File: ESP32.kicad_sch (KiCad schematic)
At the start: 4 parts, among them U1 ESP32-S3

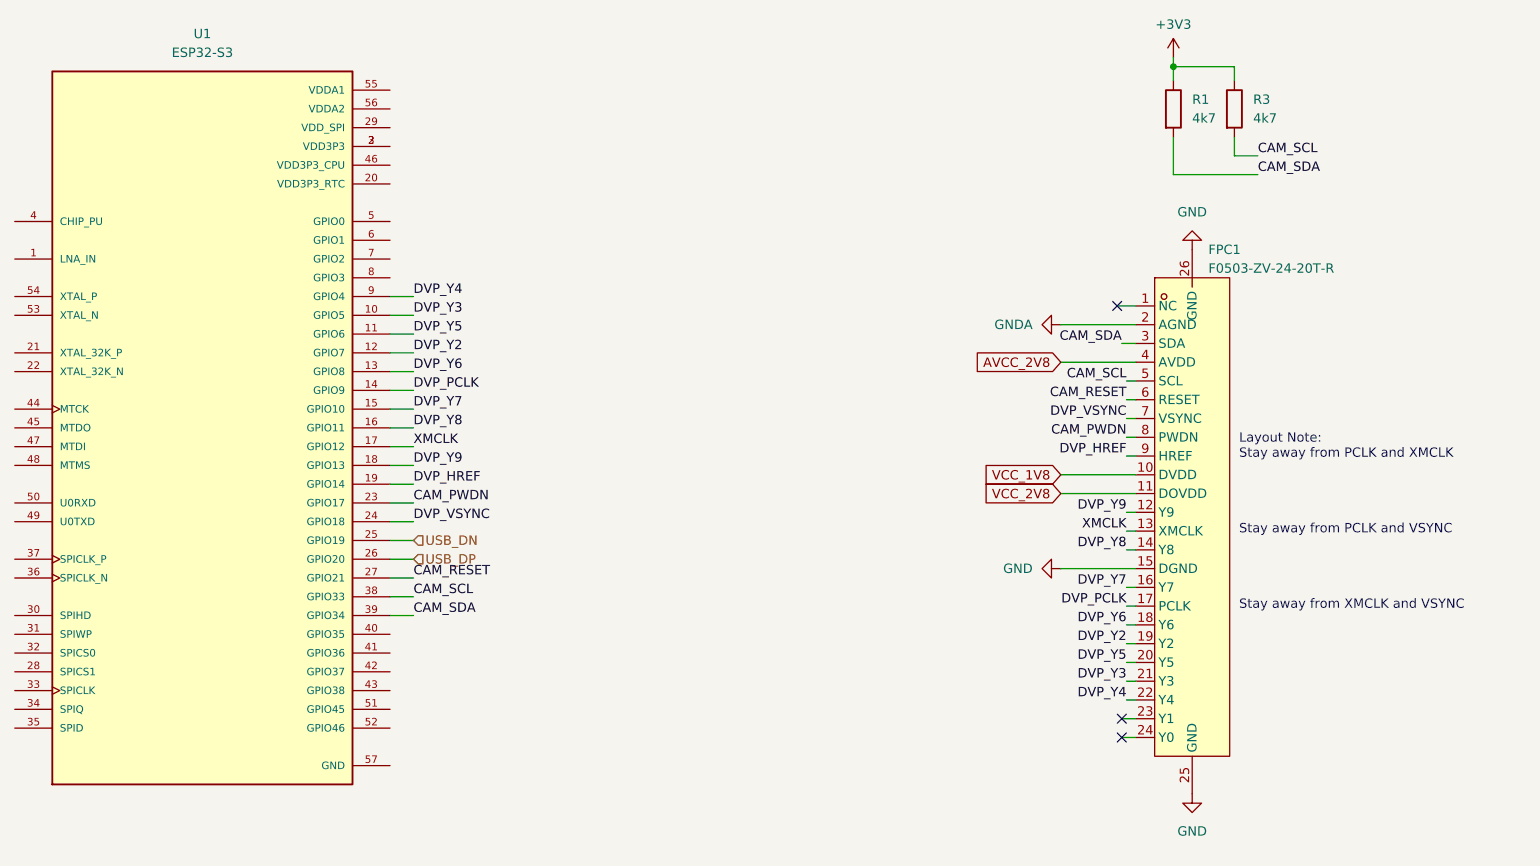
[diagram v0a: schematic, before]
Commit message: revving up
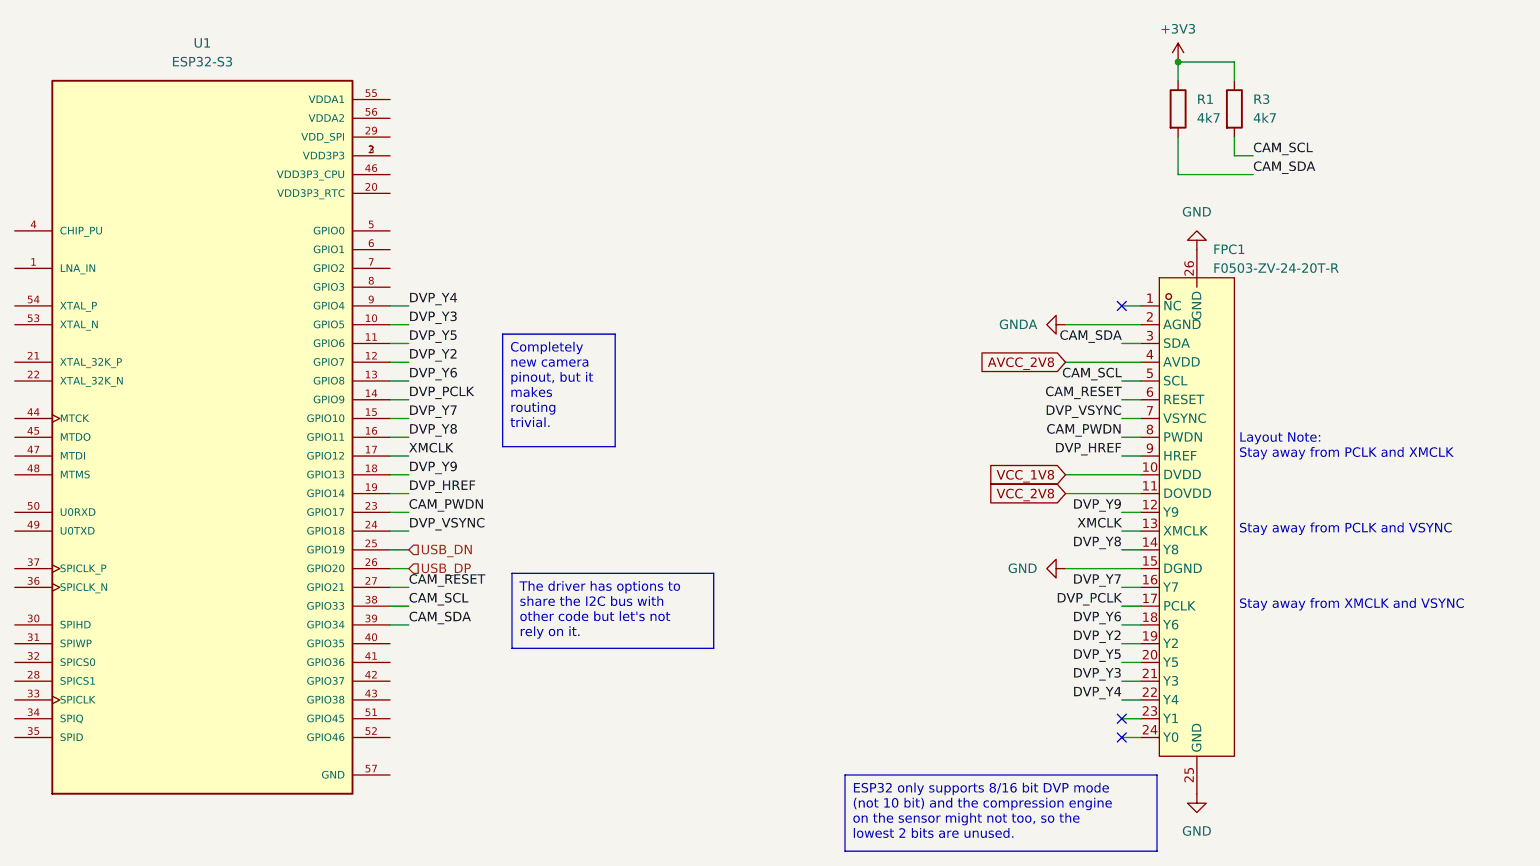
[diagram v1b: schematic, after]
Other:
- moved on the sheet: FPC1, R1, U1
